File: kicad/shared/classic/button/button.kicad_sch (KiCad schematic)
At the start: 8 parts, among them J1 Conn_01x03, Q1 BC547

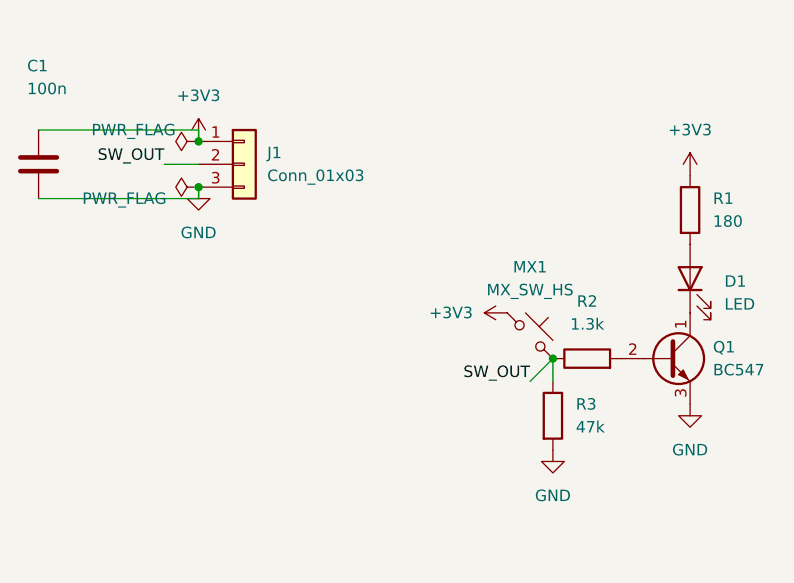
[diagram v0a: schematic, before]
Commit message: Button/LED assembly Classic actually does the thing properly now
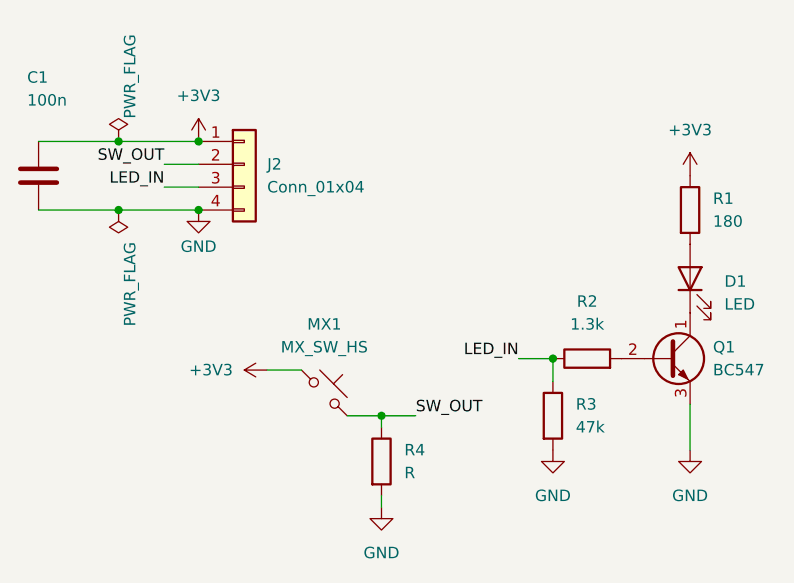
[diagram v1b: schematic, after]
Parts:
- removed J1: Conn_01x03, Connector_JST:JST_XA_S03B-XASK-1_1x03_P2.50mm_Horizontal, symbol Connector_Generic:Conn_01x03
- added J2: Conn_01x04, Connector_JST:JST_XA_B04B-XASK-1-A_1x04_P2.50mm_Vertical, symbol Connector_Generic:Conn_01x04
- added R4: R, Resistor_SMD:R_0805_2012Metric, symbol Device:R
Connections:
- net +3V3: now also J2.1 (Pin_1)
- net GND: now also J2.4 (Pin_4), R4.2
- net SW_OUT: now also J2.2 (Pin_2), R4.1; no longer R2.1, R3.1
- new net LED_IN: J2.3 (Pin_3), R2.1, R3.1
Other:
- moved on the sheet: C1, MX1
